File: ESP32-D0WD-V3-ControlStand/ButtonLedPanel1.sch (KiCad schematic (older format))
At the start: 24 parts, among them P8 CONN_5, SW10 SW_PUSH_SMALL, SW11 SW_PUSH_SMALL, SW12 SW_PUSH_SMALL, SW13 SW_PUSH_SMALL, SW14 SW_PUSH_SMALL, SW7 SW_PUSH_SMALL, SW8 SW_PUSH_SMALL, SW9 SW_PUSH_SMALL, T1 Buttons, T2 LEDS, U1 MCP23017, U2 TBD62083A

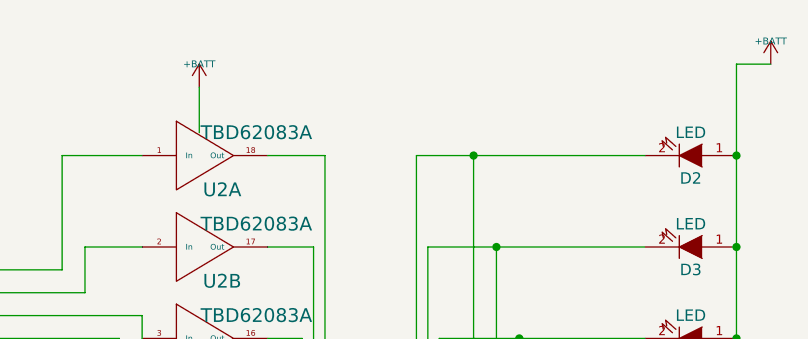
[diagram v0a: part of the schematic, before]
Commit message: Working on the PCB Layout.
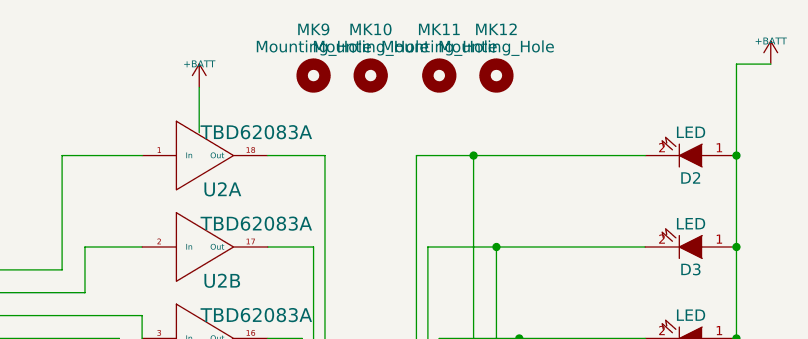
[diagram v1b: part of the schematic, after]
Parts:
- added MK10, MK11, MK12, MK9: Mounting_Hole, Mounting_Holes:MountingHole_2.5mm, symbol Mounting_Hole
- SW7, SW8, SW9: footprint Buttons_Switches_THT:SW_PUSH_6m -> Buttons_Switches_THT:SW_PUSH_6mm
- U2: footprint ~ -> Housings_SOIC:SOIC-18W_7.5x11.6mm_Pitch1.27mm
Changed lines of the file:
@@
 LIBS:mcp73871
 LIBS:lm2574n-5
+LIBS:mechanical
+LIBS:graphic_symbols
 LIBS:ESP32-D0WD-V3-ControlStand-cache
 EELAYER 25 0
@@
 F 0 "U2" H 8100 1300 60  0000 C CNN
 F 1 "TBD62083A" H 8250 1550 60  0000 C CNN
-F 2 "~" H 8000 1450 60  0000 C CNN
+F 2 "Housings_SOIC:SOIC-18W_7.5x11.6mm_Pitch1.27mm" H 8000 1450 60  0001 C CNN
 F 3 "~" H 8000 1450 60  0000 C CNN
 	2    8000 1450
@@
 F 0 "U2" H 8100 1700 60  0000 C CNN
 F 1 "TBD62083A" H 8250 1950 60  0000 C CNN
-F 2 "~" H 8000 1850 60  0000 C CNN
+F 2 "Housings_SOIC:SOIC-18W_7.5x11.6mm_Pitch1.27mm" H 8000 1850 60  0001 C CNN
 F 3 "~" H 8000 1850 60  0000 C CNN
 	3    8000 1850
@@
 F 0 "U2" H 8100 2100 60  0000 C CNN
 F 1 "TBD62083A" H 8250 2350 60  0000 C CNN
-F 2 "~" H 8000 2250 60  0000 C CNN
+F 2 "Housings_SOIC:SOIC-18W_7.5x11.6mm_Pitch1.27mm" H 8000 2250 60  0001 C CNN
 F 3 "~" H 8000 2250 60  0000 C CNN
 	4    8000 2250
@@
 F 0 "U2" H 8100 2450 60  0000 C CNN
 F 1 "TBD62083A" H 8250 2700 60  0000 C CNN
-F 2 "~" H 8000 2600 60  0000 C CNN
+F 2 "Housings_SOIC:SOIC-18W_7.5x11.6mm_Pitch1.27mm" H 8000 2600 60  0001 C CNN
 F 3 "~" H 8000 2600 60  0000 C CNN
 	5    8000 2600
@@
 F 0 "U2" H 8100 2850 60  0000 C CNN
 F 1 "TBD62083A" H 8250 3100 60  0000 C CNN
-F 2 "~" H 8000 3000 60  0000 C CNN
+F 2 "Housings_SOIC:SOIC-18W_7.5x11.6mm_Pitch1.27mm" H 8000 3000 60  0001 C CNN
 F 3 "~" H 8000 3000 60  0000 C CNN
 	6    8000 3000
@@
 F 0 "U2" H 8100 3250 60  0000 C CNN
 F 1 "TBD62083A" H 8250 3500 60  0000 C CNN
-F 2 "~" H 8000 3400 60  0000 C CNN
+F 2 "Housings_SOIC:SOIC-18W_7.5x11.6mm_Pitch1.27mm" H 8000 3400 60  0001 C CNN
 F 3 "~" H 8000 3400 60  0000 C CNN
 	7    8000 3400
@@
 F 0 "U2" H 8100 3650 60  0000 C CNN
 F 1 "TBD62083A" H 8250 3900 60  0000 C CNN
-F 2 "~" H 8000 3800 60  0000 C CNN
+F 2 "Housings_SOIC:SOIC-18W_7.5x11.6mm_Pitch1.27mm" H 8000 3800 60  0001 C CNN
 F 3 "~" H 8000 3800 60  0000 C CNN
 	8    8000 3800
@@
 F 0 "SW7" H 5900 3510 30  0000 C CNN
 F 1 "SW_PUSH_SMALL" H 5750 3321 30  0000 C CNN
-F 2 "Buttons_Switches_THT:SW_PUSH_6m" H 5750 3400 60  0001 C CNN
+F 2 "Buttons_Switches_THT:SW_PUSH_6mm" H 5750 3400 60  0001 C CNN
 F 3 "~" H 5750 3400 60  0000 C CNN
 F 4 "179-TS026660BK160LCR" H 5750 3400 60  0001 C CNN "Mouser Part Number"
@@
 F 0 "SW9" H 6100 3310 30  0000 C CNN
 F 1 "SW_PUSH_SMALL" H 5950 3121 30  0000 C CNN
-F 2 "Buttons_Switches_THT:SW_PUSH_6m" H 5950 3200 60  0001 C CNN
+F 2 "Buttons_Switches_THT:SW_PUSH_6mm" H 5950 3200 60  0001 C CNN
 F 3 "~" H 5950 3200 60  0000 C CNN
 F 4 "179-TS026660BK160LCR" H 5950 3200 60  0001 C CNN "Mouser Part Number"
@@
 F 0 "SW8" H 6000 3410 30  0000 C CNN
 F 1 "SW_PUSH_SMALL" H 5850 3221 30  0000 C CNN
-F 2 "Buttons_Switches_THT:SW_PUSH_6m" H 5850 3300 60  0001 C CNN
+F 2 "Buttons_Switches_THT:SW_PUSH_6mm" H 5850 3300 60  0001 C CNN
 F 3 "~" H 5850 3300 60  0000 C CNN
 F 4 "179-TS026660BK160LCR" H 5850 3300 60  0001 C CNN "Mouser Part Number"
@@
 	5950 3400 5950 3650
 $Comp
-L GND-RESCUE-ESP32ControlStand #PWR25
+L GND-RESCUE-ESP32ControlStand #PWR018
 U 1 1 62DF1D4E
 P 5950 3650
-F 0 "#PWR25" H 5950 3650 30  0001 C CNN
+F 0 "#PWR018" H 5950 3650 30  0001 C CNN
 F 1 "GND" H 5950 3580 30  0001 C CNN
 F 2 "" H 5950 3650 60  0000 C CNN
@@
 $EndComp
 $Comp
-L +BATT #PWR26
+L +BATT #PWR019
 U 1 1 62DF1D58
 P 8000 750
-F 0 "#PWR26" H 8000 700 20  0001 C CNN
+F 0 "#PWR019" H 8000 700 20  0001 C CNN
 F 1 "+BATT" H 8000 850 30  0000 C CNN
 F 2 "" H 8000 750 60  0000 C CNN
@@
 $EndComp
 $Comp
-L GND-RESCUE-ESP32ControlStand #PWR27
+L GND-RESCUE-ESP32ControlStand #PWR020
 U 1 1 62DF1D59
 P 8000 4200
-F 0 "#PWR27" H 8000 4200 30  0001 C CNN
+F 0 "#PWR020" H 8000 4200 30  0001 C CNN
 F 1 "GND" H 8000 4130 30  0001 C CNN
 F 2 "" H 8000 4200 60  0000 C CNN
@@
 $EndComp
 $Comp
-L +BATT #PWR28
+L +BATT #PWR021
 U 1 1 62DF1D5A
 P 10500 650
-F 0 "#PWR28" H 10500 600 20  0001 C CNN
+F 0 "#PWR021" H 10500 600 20  0001 C CNN
 F 1 "+BATT" H 10500 750 30  0000 C CNN
 F 2 "" H 10500 650 60  0000 C CNN
@@
 Connection ~ 10350 1050
 $Comp
-L GND-RESCUE-ESP32ControlStand #PWR23
+L GND-RESCUE-ESP32ControlStand #PWR022
 U 1 1 62DF1D5B
 P 4000 3850
-F 0 "#PWR23" H 4000 3850 30  0001 C CNN
+F 0 "#PWR022" H 4000 3850 30  0001 C CNN
 F 1 "GND" H 4000 3780 30  0001 C CNN
 F 2 "" H 4000 3850 60  0000 C CNN
@@
 	4000 3650 4000 3850
 $Comp
-L +3.3V-RESCUE-ESP32ControlStand #PWR24
+L +3.3V-RESCUE-ESP32ControlStand #PWR023
 U 1 1 62DF1D5C
 P 4100 1000
-F 0 "#PWR24" H 4100 960 30  0001 C CNN
+F 0 "#PWR023" H 4100 960 30  0001 C CNN
 F 1 "+3.3V" H 4100 1110 30  0000 C CNN
 F 2 "" H 4100 1000 60  0000 C CNN
@@
 Connection ~ 3400 1950
 $Comp
-L GND-RESCUE-ESP32ControlStand #PWR22
+L GND-RESCUE-ESP32ControlStand #PWR024
 U 1 1 62DF1D5D
 P 3400 2200
-F 0 "#PWR22" H 3400 2200 30  0001 C CNN
+F 0 "#PWR024" H 3400 2200 30  0001 C CNN
 F 1 "GND" H 3400 2130 30  0001 C CNN
 F 2 "" H 3400 2200 60  0000 C CNN
@@
 $EndComp
 $Comp
-L +3.3V-RESCUE-ESP32ControlStand #PWR18
+L +3.3V-RESCUE-ESP32ControlStand #PWR025
 U 1 1 62DF1D5F
 P 2600 2850
-F 0 "#PWR18" H 2600 2810 30  0001 C CNN
+F 0 "#PWR025" H 2600 2810 30  0001 C CNN
 F 1 "+3.3V" H 2600 2960 30  0000 C CNN
 F 2 "" H 2600 2850 60  0000 C CNN
@@
 $EndComp
 $Comp
-L +BATT #PWR19
+L +BATT #PWR026
 U 1 1 62DF1D61
 P 2750 1400
-F 0 "#PWR19" H 2750 1350 20  0001 C CNN
+F 0 "#PWR026" H 2750 1350 20  0001 C CNN
 F 1 "+BATT" H 2750 1500 30  0000 C CNN
 F 2 "" H 2750 1400 60  0000 C CNN
@@
 $EndComp
 $Comp
-L +3.3V-RESCUE-ESP32ControlStand #PWR20
+L +3.3V-RESCUE-ESP32ControlStand #PWR027
 U 1 1 62DF1D62
 P 2750 1550
-F 0 "#PWR20" H 2750 1510 30  0001 C CNN
+F 0 "#PWR027" H 2750 1510 30  0001 C CNN
 F 1 "+3.3V" H 2750 1660 30  0000 C CNN
 F 2 "" H 2750 1550 60  0000 C CNN
@@
 $EndComp
 $Comp
-L GND-RESCUE-ESP32ControlStand #PWR21
+L GND-RESCUE-ESP32ControlStand #PWR028
 U 1 1 62DF1D63
 P 2800 1700
-F 0 "#PWR21" H 2800 1700 30  0001 C CNN
+F 0 "#PWR028" H 2800 1700 30  0001 C CNN
 F 1 "GND" H 2800 1630 30  0001 C CNN
 F 2 "" H 2800 1700 60  0000 C CNN
@@
 	2750 2150 3400 2150
 Connection ~ 3400 2150
+$Comp
+L Mounting_Hole MK9
+U 1 1 62E6E9BE
+P 8500 700
+F 0 "MK9" H 8500 900 50  0000 C CNN
+F 1 "Mounting_Hole" H 8500 825 50  0000 C CNN
+F 2 "Mounting_Holes:MountingHole_2.5mm" H 8500 700 50  0001 C CNN
+F 3 "" H 8500 700 50  0001 C CNN
+	1    8500 700
+	1    0    0    -1
+$EndComp
+$Comp
+L Mounting_Hole MK10
+U 1 1 62E6EA13
+P 8750 700
+F 0 "MK10" H 8750 900 50  0000 C CNN
+F 1 "Mounting_Hole" H 8750 825 50  0000 C CNN
+F 2 "Mounting_Holes:MountingHole_2.5mm" H 8750 700 50  0001 C CNN
+F 3 "" H 8750 700 50  0001 C CNN
+	1    8750 700
+	1    0    0    -1
+$EndComp
+$Comp
+L Mounting_Hole MK11
+U 1 1 62E6EA6A
+P 9050 700
+F 0 "MK11" H 9050 900 50  0000 C CNN
+F 1 "Mounting_Hole" H 9050 825 50  0000 C CNN
+F 2 "Mounting_Holes:MountingHole_2.5mm" H 9050 700 50  0001 C CNN
+F 3 "" H 9050 700 50  0001 C CNN
+	1    9050 700
+	1    0    0    -1
+$EndComp
+$Comp
+L Mounting_Hole MK12
+U 1 1 62E6EAD3
+P 9300 700
+F 0 "MK12" H 9300 900 50  0000 C CNN
+F 1 "Mounting_Hole" H 9300 825 50  0000 C CNN
+F 2 "Mounting_Holes:MountingHole_2.5mm" H 9300 700 50  0001 C CNN
+F 3 "" H 9300 700 50  0001 C CNN
+	1    9300 700
+	1    0    0    -1
+$EndComp
 $EndSCHEMATC
